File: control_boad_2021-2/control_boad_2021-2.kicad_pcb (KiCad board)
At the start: 2 copper layers, 6 parts, among them J1 Conn_01x10_Female, J2 Conn_01x10_Female, J3 Conn_01x02, U1 ESP32-DevKitC, U2 IM920s

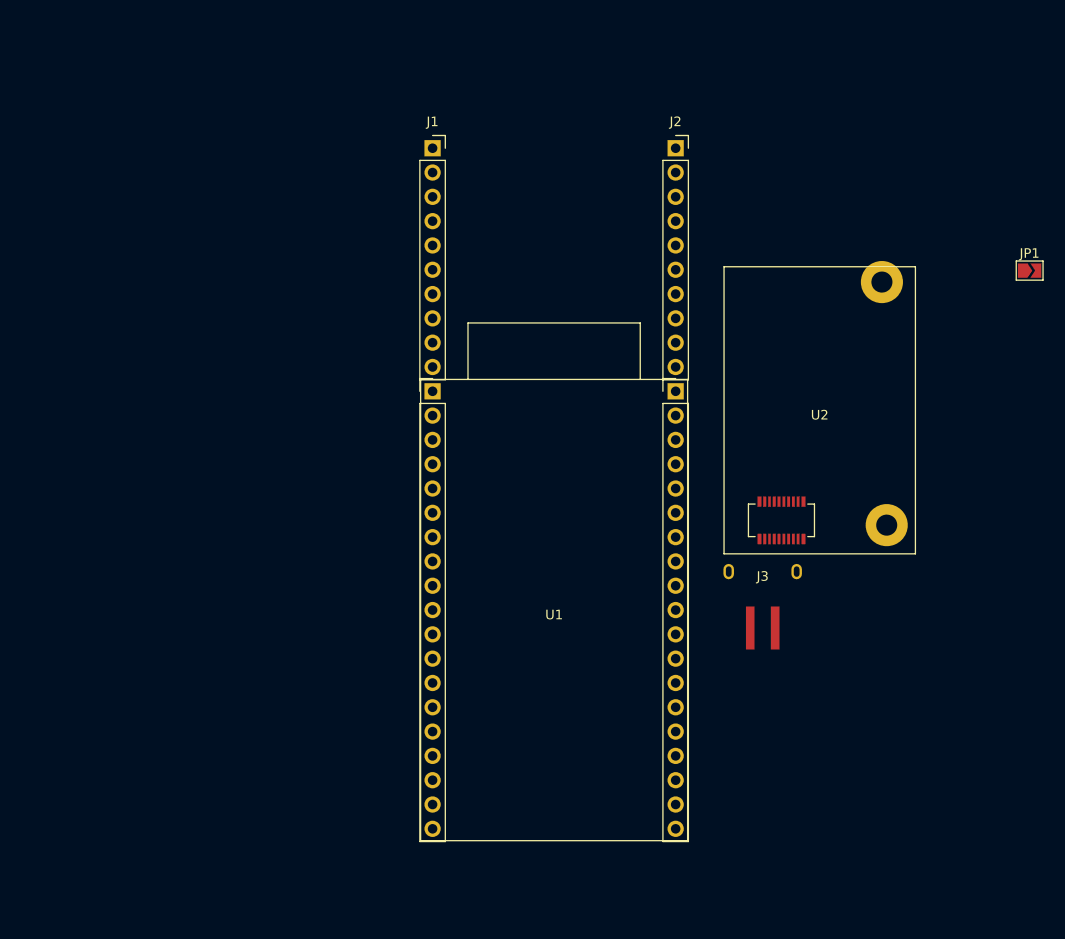
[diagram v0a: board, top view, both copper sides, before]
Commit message: complete!!!
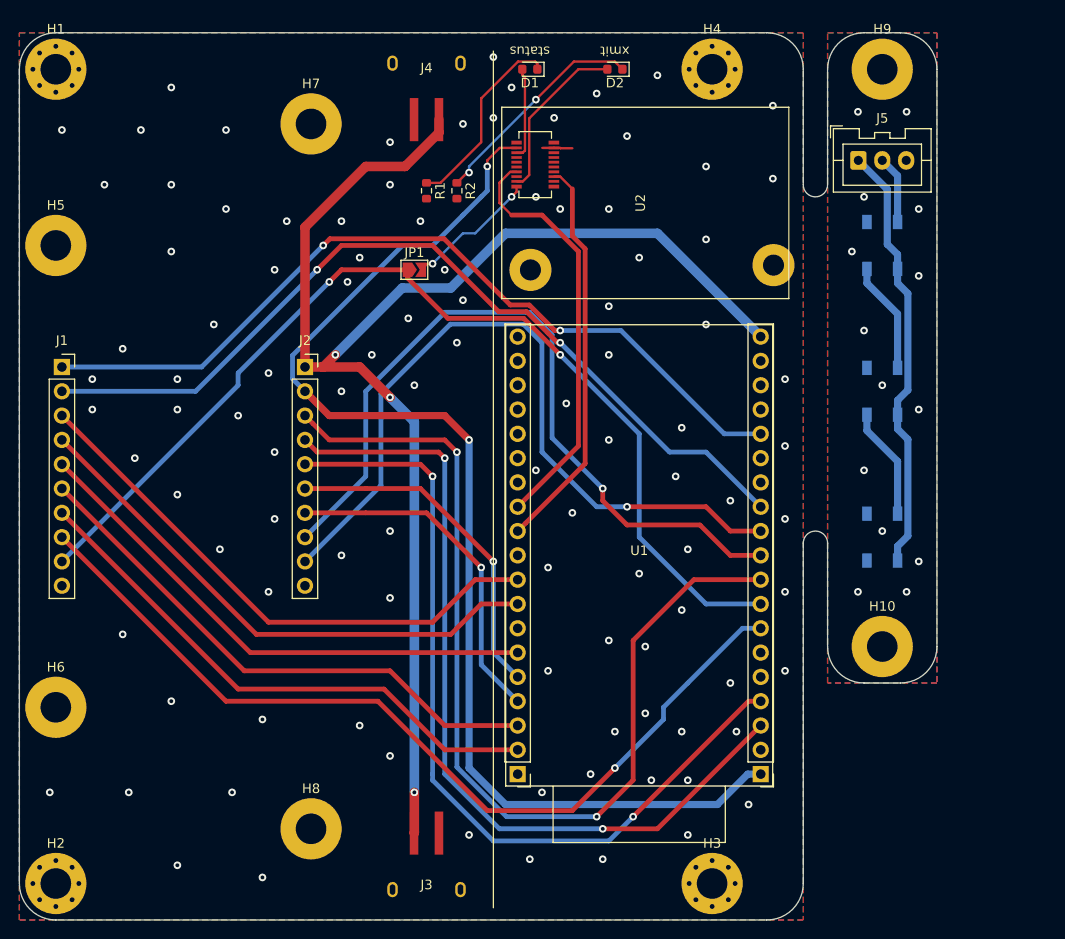
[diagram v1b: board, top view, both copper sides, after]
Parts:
- added D1: LED, LED_SMD:LED_0603_1608Metric, F.Cu at (118.7, 57.8)
- added D2: LED, LED_SMD:LED_0603_1608Metric, F.Cu at (127.6, 57.8)
- added D3: WS2812B, LED_SMD:LED_WS2812B_PLCC4_5.0x5.0mm_P3.2mm, B.Cu at (155.6, 76.2)
- added D4: WS2812B, LED_SMD:LED_WS2812B_PLCC4_5.0x5.0mm_P3.2mm, B.Cu at (155.6, 91.4)
- added D5: WS2812B, LED_SMD:LED_WS2812B_PLCC4_5.0x5.0mm_P3.2mm, B.Cu at (155.6, 106.7)
- added H1: MountingHole, MountingHole:MountingHole_3.2mm_M3_Pad_Via, F.Cu at (69.2, 57.8)
- added H10: MountingHole, MountingHole:MountingHole_3.2mm_M3_Pad, F.Cu at (155.6, 118.1)
- added H2: MountingHole, MountingHole:MountingHole_3.2mm_M3_Pad_Via, F.Cu at (69.2, 142.9)
- added H3: MountingHole, MountingHole:MountingHole_3.2mm_M3_Pad_Via, F.Cu at (137.8, 142.9)
- added H4: MountingHole, MountingHole:MountingHole_3.2mm_M3_Pad_Via, F.Cu at (137.8, 57.8)
- added H5: MountingHole_Pad, MountingHole:MountingHole_3.2mm_M3_Pad, F.Cu at (69.2, 76.2)
- added H6: MountingHole_Pad, MountingHole:MountingHole_3.2mm_M3_Pad, F.Cu at (69.2, 124.5)
- added H7: MountingHole_Pad, MountingHole:MountingHole_3.2mm_M3_Pad, F.Cu at (95.9, 63.5)
- added H8: MountingHole_Pad, MountingHole:MountingHole_3.2mm_M3_Pad, F.Cu at (95.9, 137.2)
- added H9: MountingHole, MountingHole:MountingHole_3.2mm_M3_Pad, F.Cu at (155.6, 57.8)
- added J4: Conn_01x02, Connector_USB_additional:USB micro B 2pin, F.Cu at (108.0, 57.1)
- added J5: Conn_01x03_Female, Connector_JST:JST_XA_B03B-XASK-1_1x03_P2.50mm_Vertical, F.Cu at (153.1, 67.3)
- added R1: R, Resistor_SMD:R_0603_1608Metric, F.Cu at (108.0, 70.5)
- added R2: R, Resistor_SMD:R_0603_1608Metric, F.Cu at (111.1, 70.5)
- moved JP1 64.3 mm to (106.7, 78.7)
- moved J3 48.4 mm to (108.0, 143.5), turned to 180 degrees
- moved J2 45.0 mm to (95.2, 88.9)
- moved J1 45.0 mm to (69.8, 88.9)
- moved U2 28.3 mm to (130.8, 71.8), turned to 270 degrees
- moved U1 10.6 mm to (130.2, 108.6), turned to 180 degrees
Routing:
- net +5V: track 0.00 -> 146.9 mm, vias 0 -> 3
- net +3V3: track 0.00 -> 125.5 mm, vias 0 -> 2
- net digital8_io33: track 0.00 -> 107.7 mm, vias 0 -> 2
- net analog0_io25: track 0.00 -> 103.1 mm, vias 0 -> 2
- net digital7_io32: track 0.00 -> 93.5 mm, vias 0 -> 1
- net digital1_io14: track 0.00 -> 90.6 mm, vias 0 -> 2
- net analog2_io39: track 0.00 -> 88.6 mm, vias 0 -> 2
- net anarog1_io36: track 0.00 -> 88.3 mm, vias 0 -> 2
- net digital0_io13: track 0.00 -> 87.0 mm, vias 0 -> 2
- net serial1_RX_io26: track 0.00 -> 80.2 mm, vias 0 -> 1
- net serial1_TX_io27: track 0.00 -> 79.2 mm, vias 0 -> 1
- net digital2_io18: track 0.00 -> 58.4 mm
- net digital6_io23: track 0.00 -> 57.9 mm
- net digital5_io22: track 0.00 -> 57.9 mm
- net digital3_io19: track 0.00 -> 57.4 mm
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- added copper zone on B.Cu, net GND
- added copper zone on F.Cu, net GND
- added copper zone on B.Cu, net GNDA
- added copper zone on F.Cu, net GNDA
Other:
- board outline added: 95.9 x 92.7 mm
- board text added: "status"
- board text added: "xmit"
